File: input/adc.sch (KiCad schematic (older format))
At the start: 1 part, among them U101 LTC2508IDKD-32

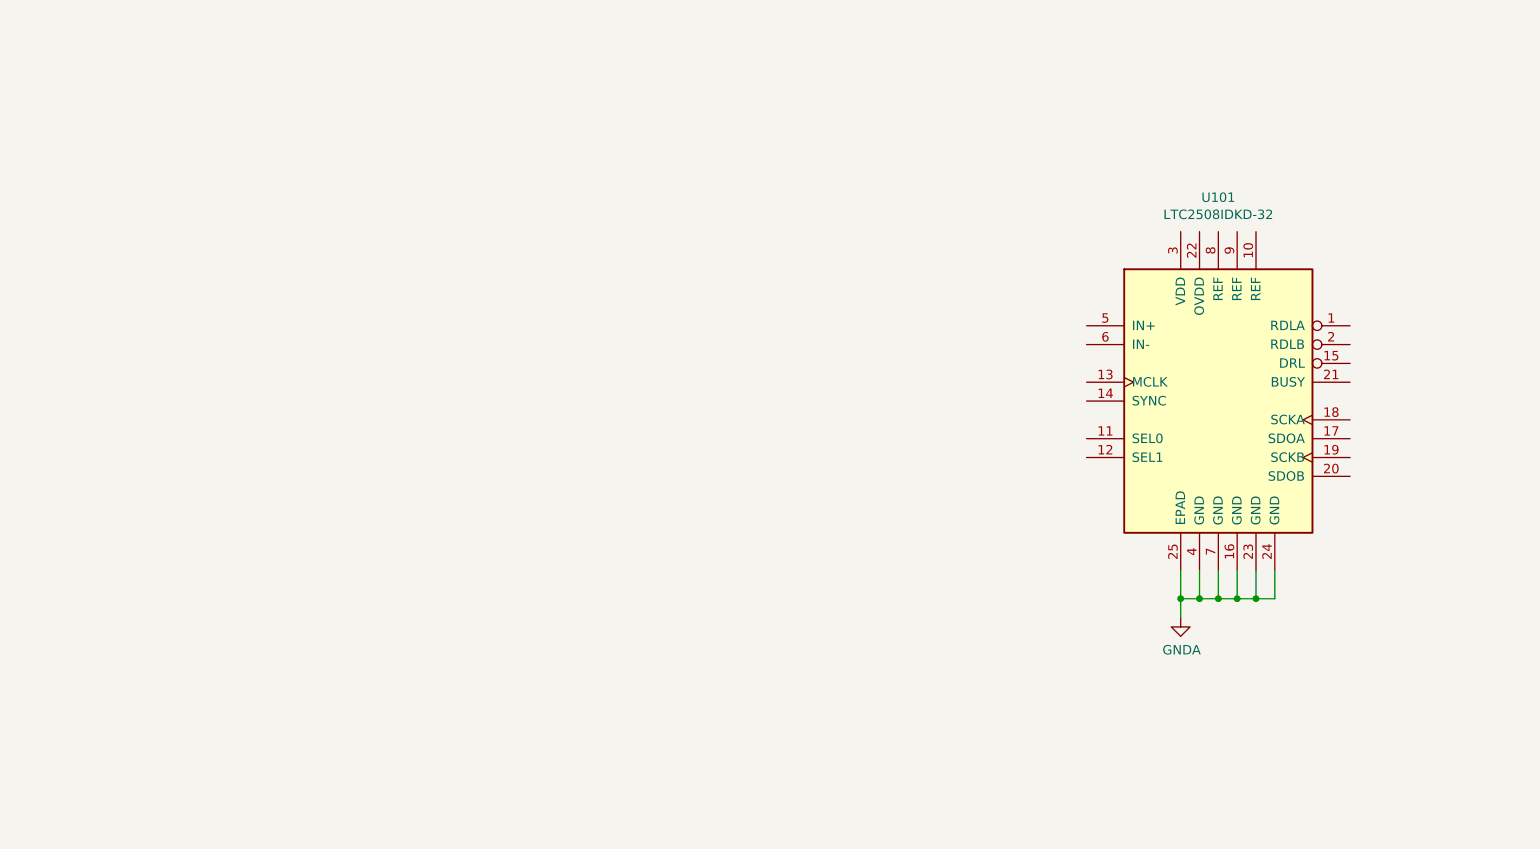
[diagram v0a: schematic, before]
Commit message: More work on input board
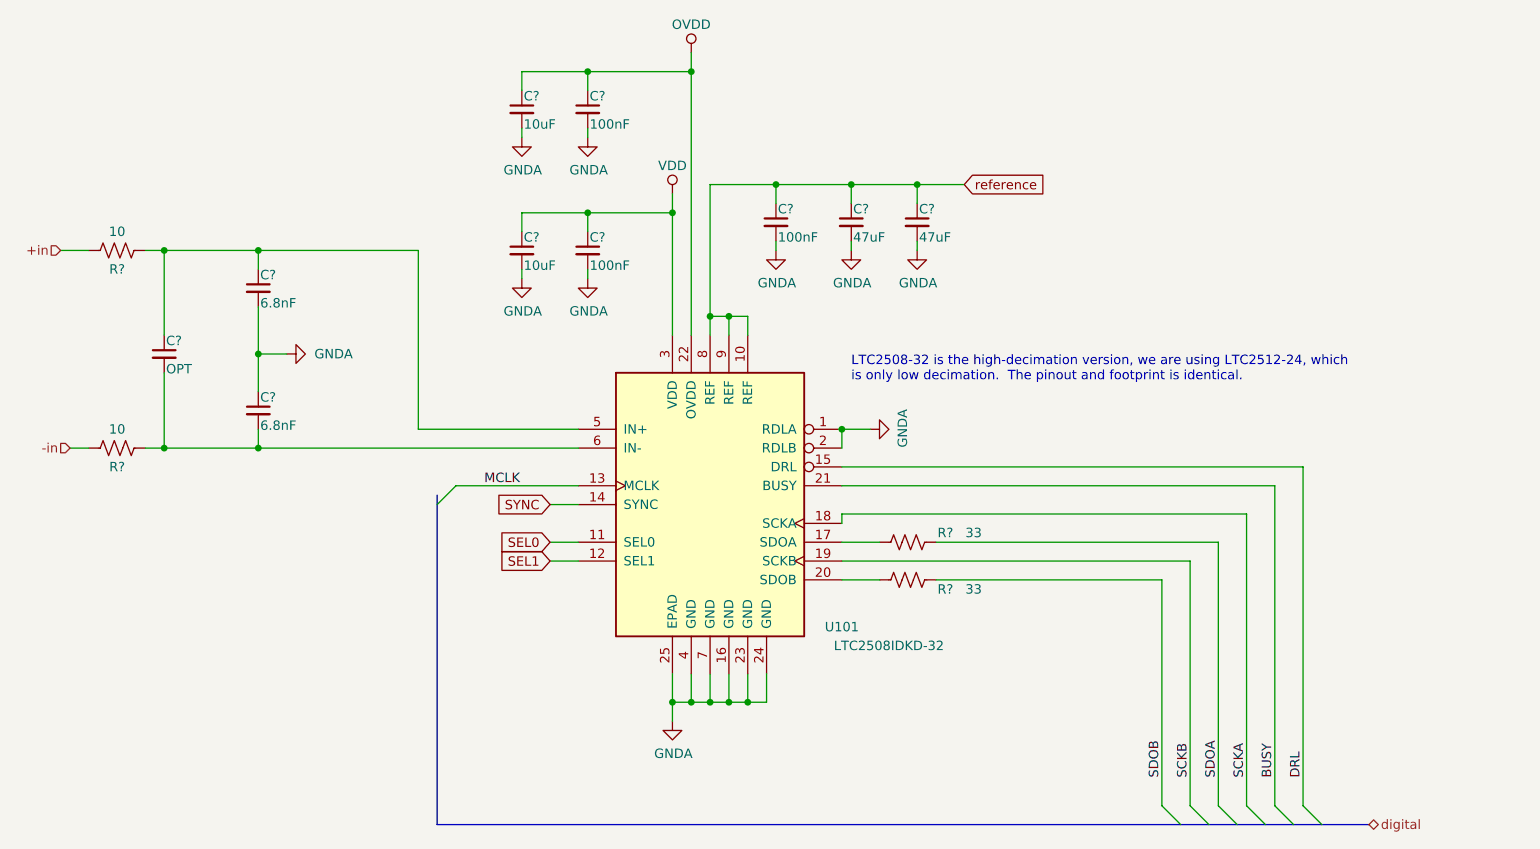
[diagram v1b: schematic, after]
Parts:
- added C? (x2): 47uF, Capacitor_SMD:C_1210_3225Metric, symbol Device:C_Small
- added C? (x2): 10uF, Capacitor_SMD:C_0603_1608Metric, symbol Device:C_Small
- added C? (x3): 100nF, Capacitor_SMD:C_0603_1608Metric, symbol Device:C_Small
- added C? (x2): 6.8nF, Capacitor_SMD:C_1206_3216Metric, symbol Device:C_Small
- added C?: OPT, Capacitor_SMD:C_1206_3216Metric, symbol Device:C_Small
- added R? (x2): 10, symbol Device:R_US
- added R? (x2): 33, Capacitor_SMD:C_0402_1005Metric, symbol Device:R_US
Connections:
- net GNDA: now also U101.1 (RDLA), U101.2 (RDLB), C?.1, C?.2, C?.2, C?.2, C?.2, C?.2, C?.2, C?.2, C?.2
- net reference: now reaches U101.10 (REF)
- net reference: now also U101.8 (REF), U101.9 (REF), C?.1, C?.1, C?.1
- net SEL0: now reaches U101.11 (SEL0)
- net SEL1: now reaches U101.12 (SEL1)
- net MCLK: now reaches U101.13 (MCLK)
- net SYNC: now reaches U101.14 (SYNC)
- net DRL: now reaches U101.15 (DRL)
- net at U101.17 (SDOA): now also R?.2
- net SCKA: now reaches U101.18 (SCKA)
- net SCKB: now reaches U101.19 (SCKB)
- net at U101.20 (SDOB): now also R?.2
- net BUSY: now reaches U101.21 (BUSY)
- net OVDD: now reaches U101.22 (OVDD)
- net OVDD: now also C?.1, C?.1
- net VDD: now reaches U101.3 (VDD)
- net VDD: now also C?.1, C?.1
- net at U101.5 (IN+): now also C?.1, C?.1, R?.1
- net at U101.6 (IN-): now also C?.2, C?.2, R?.1
- new net +in: R?.2
- new net -in: R?.2
- new net SDOA: R?.1
- new net SDOB: R?.1
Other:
- note added: "LTC2508-32 is the high-decimation version, we are using LTC2512-24, which\nis only low decimation. The pinout and footprint is identical."
- moved on the sheet: U101
